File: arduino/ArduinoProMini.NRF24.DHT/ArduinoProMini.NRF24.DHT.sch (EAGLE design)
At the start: 8 parts, among them U1 DHT22

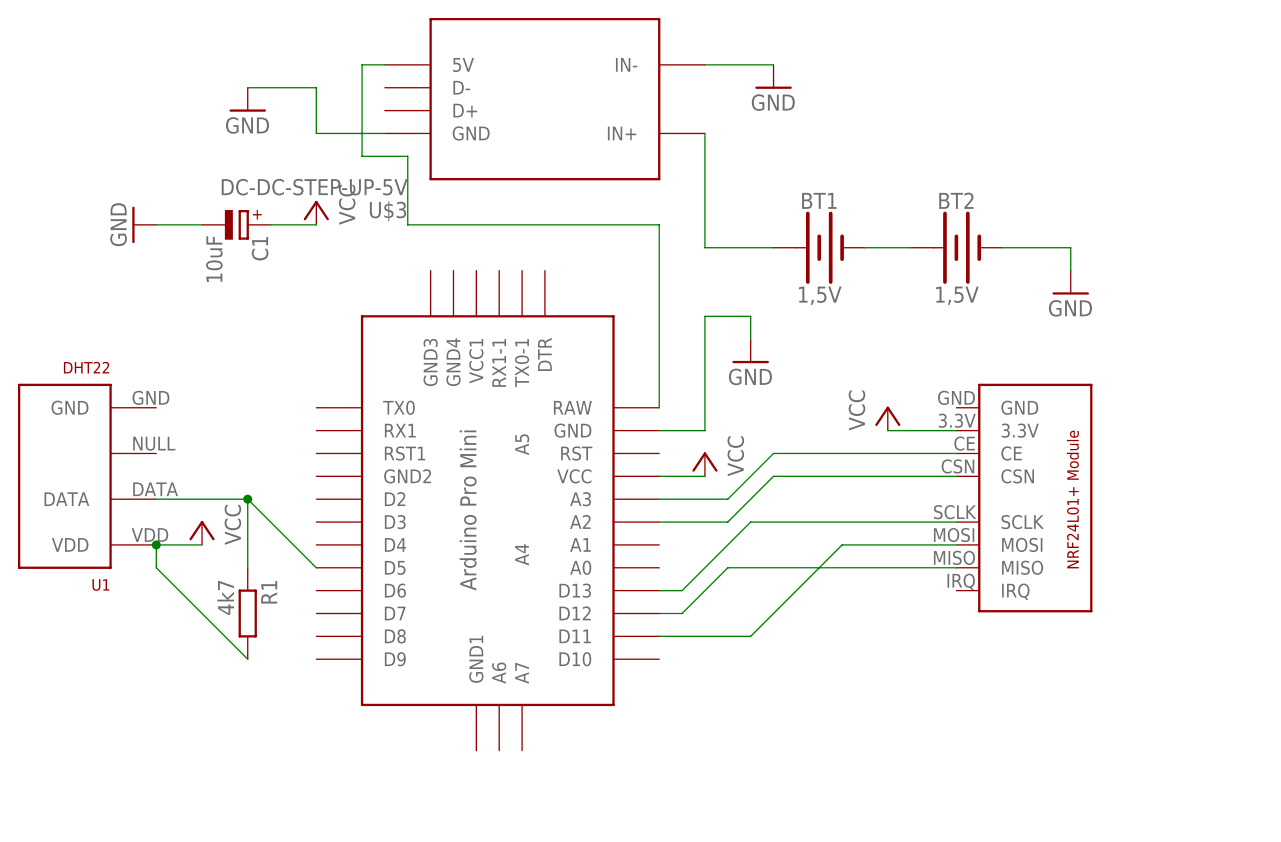
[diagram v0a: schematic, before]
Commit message: added schematic + board
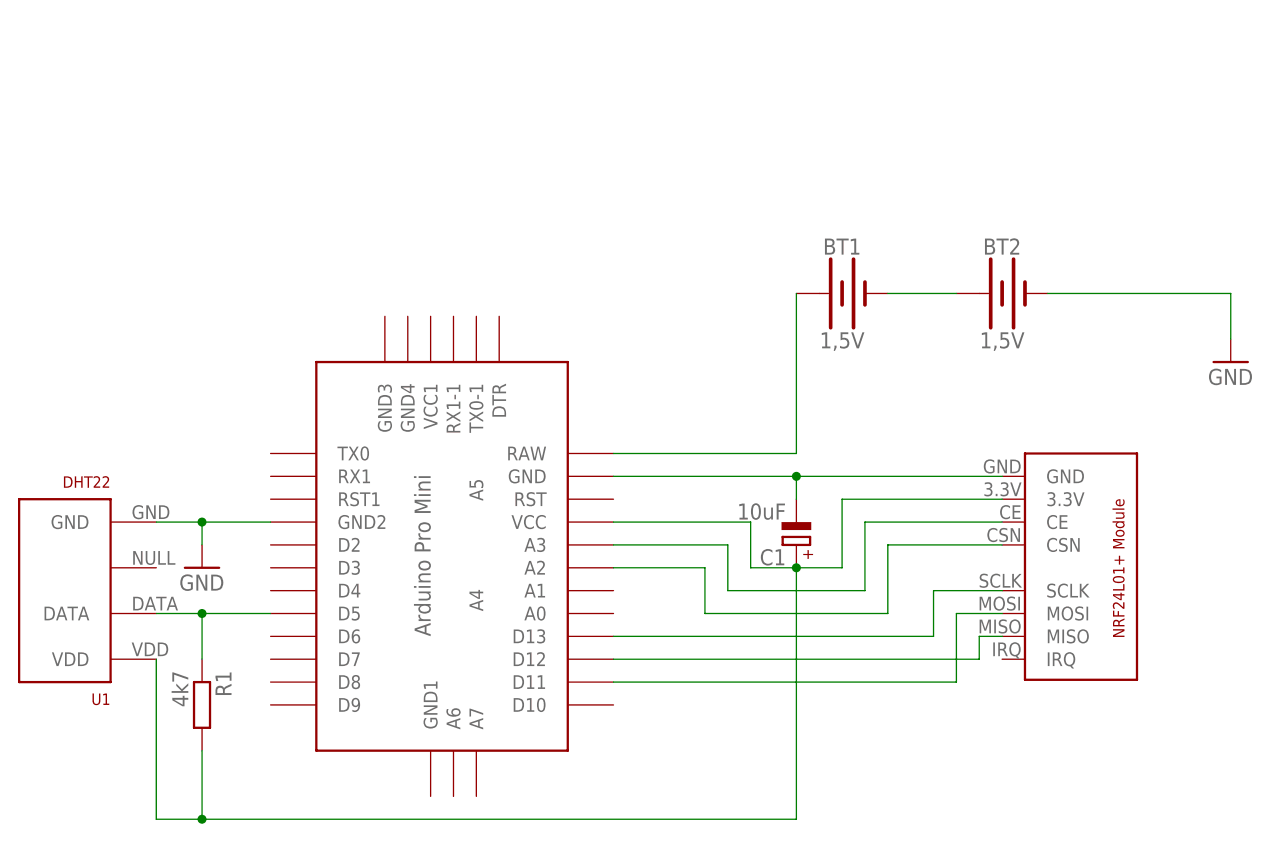
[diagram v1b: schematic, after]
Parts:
- removed U$3: DC-DC-STEP-UP-5V, diy-modules:DC-DC-STEP-UP-5V
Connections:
- net VCC renamed 3.3V
- removed net N$2 (its old number): BT1.+, U$3.IN+
- removed net N$9 (its old number): U$1.RAW, U$3.5V
- new net RAW: BT1.+, U$1.RAW
- net GND: now also U$1.GND2, U$2.GND, U1.GND; no longer U$3.GND, U$3.IN-
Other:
- moved on the sheet: BT1, BT2, C1, R1, U1
